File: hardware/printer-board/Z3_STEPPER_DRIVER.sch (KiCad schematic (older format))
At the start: 9 parts, among them J13 MS_SELECT, J14 Z3, U8 A4988_MODULE

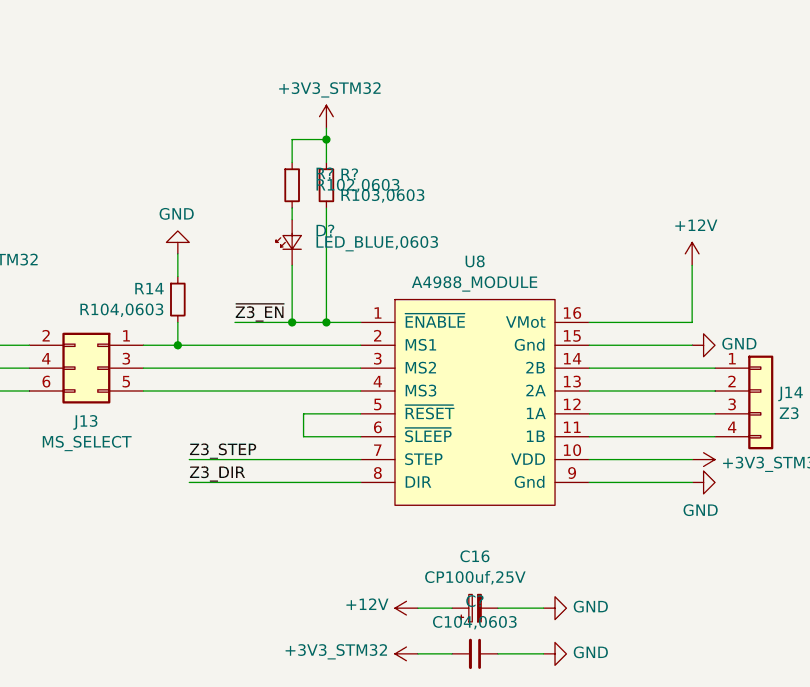
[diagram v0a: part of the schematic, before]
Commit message: update annotations,
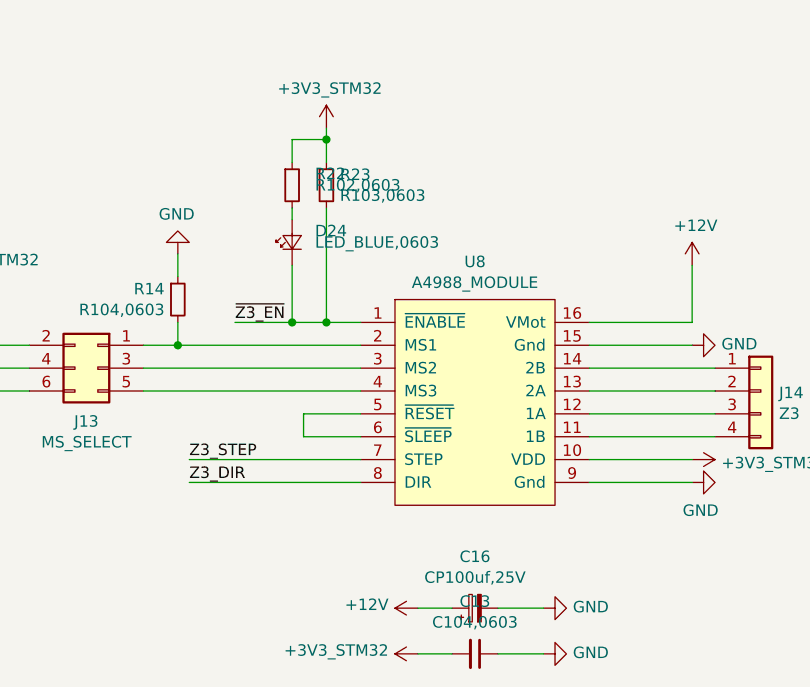
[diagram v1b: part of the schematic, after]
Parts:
- gave numbers to parts that had none: 4
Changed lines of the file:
@@
 $EndBitmap
 $Comp
-L taobao-components:+3V3_STM32 #PWR?
+L taobao-components:+3V3_STM32 #PWR023
 U 1 1 5CC40ABB
 P 3500 2700
-F 0 "#PWR?" H 3500 2550 50  0001 C CNN
+F 0 "#PWR023" H 3500 2550 50  0001 C CNN
 F 1 "+3V3_STM32" H 3515 2873 50  0000 C CNN
 F 2 "" H 3500 2700 50  0001 C CNN
@@
 $EndComp
 $Comp
-L taobao-components:+3V3_STM32 #PWR?
+L taobao-components:+3V3_STM32 #PWR025
 U 1 1 5CC40AD2
 P 5400 4250
-F 0 "#PWR?" H 5400 4100 50  0001 C CNN
+F 0 "#PWR025" H 5400 4100 50  0001 C CNN
 F 1 "+3V3_STM32" V 5415 4378 50  0000 L CNN
 F 2 "" H 5400 4250 50  0001 C CNN
@@
 $EndComp
 $Comp
-L taobao-components:+3V3_STM32 #PWR?
+L taobao-components:+3V3_STM32 #PWR024
 U 1 1 5CC40AFB
 P 6600 3400
-F 0 "#PWR?" H 6600 3250 50  0001 C CNN
+F 0 "#PWR024" H 6600 3250 50  0001 C CNN
 F 1 "+3V3_STM32" V 6615 3528 50  0000 L CNN
 F 2 "" H 6600 3400 50  0001 C CNN
@@
 $EndComp
 $Comp
-L taobao-c:C104,0603 C?
+L taobao-c:C104,0603 C13
 U 1 1 5CC40BF1
 P 5650 4250
-F 0 "C?" V 5421 4250 50  0000 C CNN
+F 0 "C13" V 5421 4250 50  0000 C CNN
 F 1 "C104,0603" V 5512 4250 50  0000 C CNN
 F 2 "Capacitor_SMD:C_0603_1608Metric_Pad1.05x0.95mm_HandSolder" H 5650 4250 50  0001 C CNN
@@
 AR Path="/5CC0A8C5/5CC5CA27" Ref="R?"  Part="1"
 AR Path="/5CC0A8CA/5CC5CA27" Ref="R?"  Part="1"
-AR Path="/5CC0A8CF/5CC5CA27" Ref="R?"  Part="1"
+AR Path="/5CC0A8CF/5CC5CA27" Ref="R23"  Part="1"
 AR Path="/5CC0AEC9/5CC5CA27" Ref="R?"  Part="1"
-F 0 "R?" H 5059 2246 50  0000 L CNN
+F 0 "R23" H 5059 2246 50  0000 L CNN
 F 1 "R103,0603" H 5059 2155 50  0000 L CNN
 F 2 "Resistor_SMD:R_0603_1608Metric_Pad1.05x0.95mm_HandSolder" H 5000 2200 50  0001 C CNN
@@
 P 5000 1950
 AR Path="/5CC0AEC9/5CC5CA2F" Ref="#PWR?"  Part="1"
-AR Path="/5CC0A8CF/5CC5CA2F" Ref="#PWR?"  Part="1"
-F 0 "#PWR?" H 5000 1800 50  0001 C CNN
+AR Path="/5CC0A8CF/5CC5CA2F" Ref="#PWR022"  Part="1"
+F 0 "#PWR022" H 5000 1800 50  0001 C CNN
 F 1 "+3V3_STM32" H 5015 2123 50  0000 C CNN
 F 2 "" H 5000 1950 50  0001 C CNN
@@
 AR Path="/5CC15C35/5CC5CA35" Ref="R?"  Part="1"
 AR Path="/5CC0AEC9/5CC5CA35" Ref="R?"  Part="1"
-AR Path="/5CC0A8CF/5CC5CA35" Ref="R?"  Part="1"
-F 0 "R?" H 4950 2250 50  0000 L CNN
+AR Path="/5CC0A8CF/5CC5CA35" Ref="R22"  Part="1"
+F 0 "R22" H 4950 2250 50  0000 L CNN
 F 1 "R102,0603" H 4950 2200 50  0000 L CNN
 F 2 "Resistor_SMD:R_0603_1608Metric_Pad1.05x0.95mm_HandSolder" H 4850 2200 50  0001 C CNN
@@
 AR Path="/5CC15C35/5CC5CA3C" Ref="D?"  Part="1"
 AR Path="/5CC0AEC9/5CC5CA3C" Ref="D?"  Part="1"
-AR Path="/5CC0A8CF/5CC5CA3C" Ref="D?"  Part="1"
-F 0 "D?" V 4900 2350 50  0000 R CNN
+AR Path="/5CC0A8CF/5CC5CA3C" Ref="D24"  Part="1"
+F 0 "D24" V 4900 2350 50  0000 R CNN
 F 1 "LED_BLUE,0603" V 4850 2350 50  0000 R CNN
 F 2 "LED_SMD:LED_0603_1608Metric_Pad1.05x0.95mm_HandSolder" V 4850 2450 50  0001 C CNN
